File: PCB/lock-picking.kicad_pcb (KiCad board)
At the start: 2 copper layers, 25 x 24 mm, 22 parts, among them U1 HX PZ2.54-1X5P ZZ, U2 DRV8876PWPR, U3 MLX90393SLW-ABA-011-RE, U4 SMTSOM225BTR, U5 S2B-PH-K-S, U6 SMTSOM225BTR, U7 HX TYPE-C 16PIN, U8 AMS1117-5.0_C347223

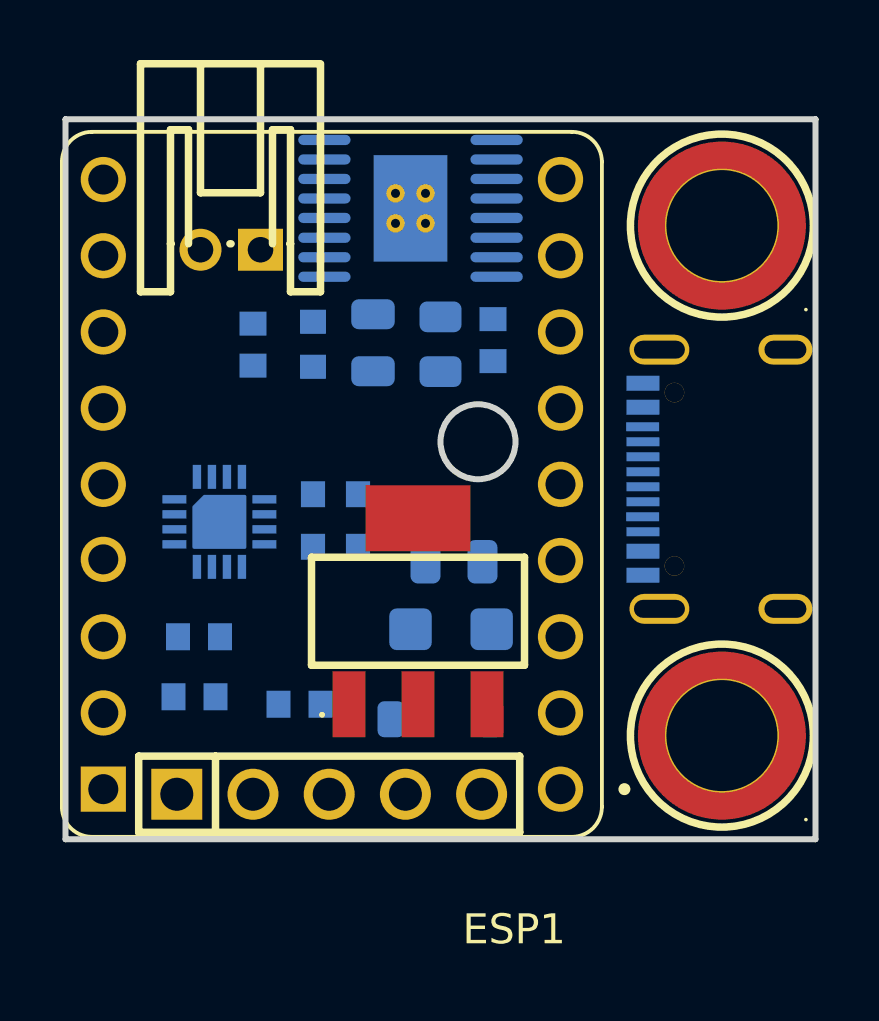
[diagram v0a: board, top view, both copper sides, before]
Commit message: PCB routing
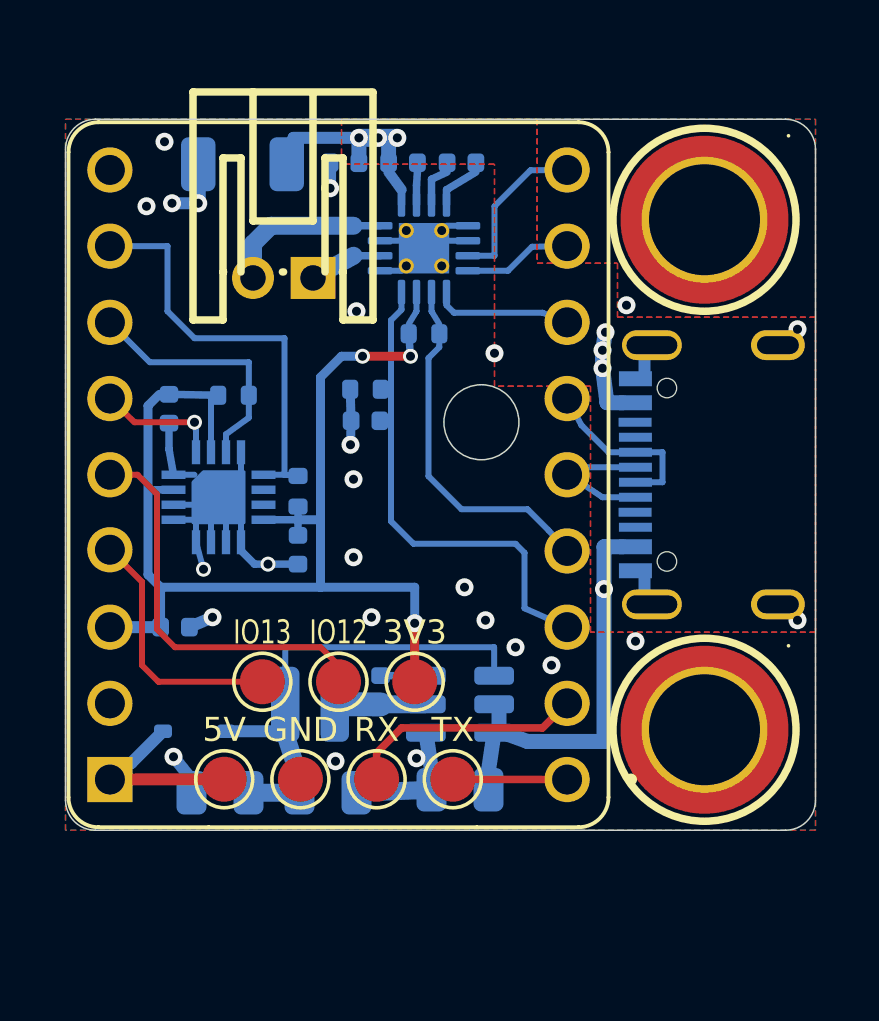
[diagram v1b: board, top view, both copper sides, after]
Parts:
- removed ESP1: ESP32-S3-SuperMini, footprints:ESP32-S3-SuperMini
- removed R5: 10, Resistor_SMD:R_0805_2012Metric
- removed U5: S2B-PH-K-S, EasyEDA:CONN-TH_S2B-PH-K-S-LF-SN
- removed U6: SMTSOM225BTR, EasyEDA:SMD_BD5.6-D3.6
- removed U7: HX TYPE-C 16PIN, EasyEDA:TYPE-C-SMD_HX-TYPE-C-16PIN
- removed U8: AMS1117-5.0_C347223, EasyEDA:SOT-223_L6.7-W3.5-P2.30-BR
- added C1: 10uF 25V, Capacitor_SMD:C_0805_2012Metric, B.Cu at (25.1, 34.4)
- added C10: 100nF 16V, Capacitor_SMD:C_0402_1005Metric, B.Cu at (19.8, 26.4)
- added C11: 10uF 6.3V, Capacitor_SMD:C_0402_1005Metric, B.Cu at (15.7, 28.9)
- added C12: 10nF 50V, Capacitor_SMD:C_0402_1005Metric, B.Cu at (22.0, 22.1)
- added H1: M2 SMD nut, Library:M2_SMD_nut_SMTSOM225_ring4.2, F.Cu at (33.3, 15.3)
- added H2: M2 SMD nut, Library:M2_SMD_nut_SMTSOM225_ring4.2, F.Cu at (33.3, 32.4)
- added J1: USB-C 16P (12V + I2C), Library:USB-C_HX-TYPE-C-16PIN_NPTH-pegs, B.Cu at (33.4, 23.9)
- added J2: Motor (JST-PH 2P), EasyEDA:CONN-TH_S2B-PH-K-S-LF-SN, F.Cu at (19.2, 17.3)
- added L1: 4.7uH, Inductor_SMD:L_Changjiang_FTC252012S, B.Cu at (20.1, 31.5)
- added R1: 1.5k 1%, Resistor_SMD:R_0402_1005Metric, B.Cu at (22.0, 21.0)
- added TP1: Pad, TestPoint:TestPoint_Pad_D1.5mm, F.Cu at (21.1, 30.8)
- added TP2: Pad, TestPoint:TestPoint_Pad_D1.5mm, F.Cu at (18.6, 30.8)
- added TP3: Pad, TestPoint:TestPoint_Pad_D1.5mm, F.Cu at (24.9, 34.0)
- added TP4: Pad, TestPoint:TestPoint_Pad_D1.5mm, F.Cu at (22.4, 34.0)
- added TP5: Pad, TestPoint:TestPoint_Pad_D1.5mm, F.Cu at (23.6, 30.8)
- added TP6: Pad, TestPoint:TestPoint_Pad_D1.5mm, F.Cu at (17.3, 34.0)
- added TP7: Pad, TestPoint:TestPoint_Pad_D1.5mm, F.Cu at (19.8, 34.0)
- C2, C9: value CC0603KRX7R9BB104 -> 100nF 16V; footprint EasyEDA:C0603 -> Capacitor_SMD:C_0402_1005Metric
- C3: value CL10B223KB8NNNC-22nF -> 47uF 6.3V; footprint EasyEDA:C0603 -> Capacitor_SMD:C_0805_2012Metric
- C4: value CC0603KRX7R9BB104 -> 47uF 6.3V; footprint EasyEDA:C0603 -> Capacitor_SMD:C_0805_2012Metric
- C5: value 10uF 25V -> 100nF 50V; footprint Capacitor_SMD:C_0805_2012Metric -> Capacitor_SMD:C_0402_1005Metric
- C6: value 10uF 16V tant -> 22uF 25V; footprint Capacitor_Tantalum_SMD:CP_EIA-3216-18_Kemet-A -> Capacitor_SMD:C_1206_3216Metric
- C7: value 10uF 25V -> 100nF 16V; footprint Capacitor_SMD:C_0805_2012Metric -> Capacitor_SMD:C_0402_1005Metric
- C8: value CC0603KRX7R9BB104 -> 22nF 50V; footprint EasyEDA:C0603 -> Capacitor_SMD:C_0402_1005Metric
- D1: value B5819W -> 1N5819WS; footprint Diode_SMD:D_SOD-123 -> Diode_SMD:D_SOD-323
- R2: value 0603WAF1501T5E -> 10k; footprint EasyEDA:R0603 -> Resistor_SMD:R_0402_1005Metric
- R3, R4: value 10k -> 2.2k; footprint EasyEDA:R0603 -> Resistor_SMD:R_0402_1005Metric
- U1: value HX PZ2.54-1X5P ZZ -> ESP32-S3-SuperMini; footprint EasyEDA:HDR-TH_5P-P2.54-V-M -> footprints:ESP32-S3-SuperMini
- U2: value DRV8876PWPR -> DRV8876RGTR; footprint EasyEDA:HTSSOP-16_L5.0-W4.4-P0.65-LS6.4-BL-EP -> Library:QFN-16-1EP_3x3mm_P0.5mm_EP1.68x1.68mm_ThermalVias0.3
- U4: value SMTSOM225BTR -> AP63205WU-7; footprint EasyEDA:SMD_BD5.6-D3.6 -> Package_TO_SOT_SMD:TSOT-23-6; moved to B.Cu
- moved C8 19.9 mm to (25.2, 13.4), turned to 0 degrees
- moved U4 18.2 mm to (25.1, 31.5), turned to 180 degrees
- moved C6 17.0 mm to (17.9, 13.5), turned to 180 degrees
- moved C3 16.1 mm to (20.8, 34.5), turned to 0 degrees
- moved C4 15.0 mm to (17.1, 34.5), turned to 180 degrees
- moved C7 13.4 mm to (23.2, 13.4)
- moved U1 10.7 mm to (21.1, 23.9), turned to 180 degrees
- moved D1 8.21 mm to (16.3, 32.4), turned to 0 degrees
- moved C9 7.67 mm to (15.4, 21.6), turned to -90 degrees
- moved R4 6.09 mm to (17.6, 21.2)
- moved C5 6.07 mm to (21.3, 13.4), turned to 180 degrees
- moved R2 3.72 mm to (23.9, 19.1), turned to 180 degrees
- moved C2 2.74 mm to (22.5, 31.0), turned to 90 degrees
- moved U2 1.40 mm to (23.9, 16.3)
- moved R3 1.25 mm to (19.8, 24.4), turned to -90 degrees
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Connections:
- C2 pad 1: 12v -> Net-(U4-SW)
- C2 pad 2: GND -> Net-(U4-BST)
- C3 pad 1: Net-(U2-CPL) -> +5V
- C3 pad 2: Net-(U2-CPH) -> GND
- C4 pad 1: Net-(U2-VCP) -> +5V
- C4 pad 2: 12v -> GND
- C5 pad 1: VIN_LDO -> +12V
- C6 pad 1: 5v -> +12V
- C7 pad 1: 12v -> /DRV_VCP
- C7 pad 2: GND -> +12V
- C8 pad 1: GND -> /DRV_CPH
- C8 pad 2: 3v3 -> /DRV_CPL
- C9 pad 1: GND -> +3V3
- C9 pad 2: 3v3 -> GND
- D1 pad 2: 5v -> +5V
- R2 pad 1: GND -> /DRV_nFAULT
- R2 pad 2: IPROPI -> +3V3
- R3 pad 1: 3v3 -> /MAG_SDA
- R3 pad 2: MAG_SDA -> +3V3
- R4 pad 1: 3v3 -> /MAG_SCL
- R4 pad 2: MAG_SCL -> +3V3
- U1 pad 1: VBUS -> /DRV_IPROPI
- U1 pad 2: GND -> /DRV_nFAULT
- U1 pad 3: GPIO9 -> /I2C_SDA
- U1 pad 4: GPIO8 -> /I2C_SCL
- U1 pad 5: GPIO7 -> /DRV_nSLEEP
- U2 pad 1: IN1 -> /DRV_nSLEEP
- U2 pad 10: Net-(U2-OUT2) -> /DRV_VCP
- U2 pad 11: 12v -> /DRV_CPH
- U2 pad 12: Net-(U2-VCP) -> /DRV_CPL
- U2 pad 13: Net-(U2-CPH) -> GND
- U2 pad 14: Net-(U2-CPL) -> GND
- U2 pad 15: GND -> /DRV_IN1_EN
- U2 pad 16: PMODE -> /DRV_IN2_PH
- U2 pad 2: IN2 -> /DRV_nFAULT
- U2 pad 3: nSLEEP -> +3V3
- U2 pad 4: nFAULT -> /DRV_IPROPI
- U2 pad 5: nSLEEP -> GND
- U2 pad 6: IPROPI -> /MOT_OUT1
- U2 pad 8: Net-(U2-OUT1) -> /MOT_OUT2
- U2 pad 9: GND -> +12V
- U3 pad 1: unconnected-(U3-INT-Pad1) -> /MAG_INT
- U3 pad 10: unconnected-(U3-N/C-Pad10) -> GND
- U3 pad 14: unconnected-(U3-N/C-Pad14) -> GND
- U3 pad 15: 3v3 -> +3V3
- U3 pad 16: unconnected-(U3-N/C-Pad16) -> GND
- U3 pad 17: unconnected-(U3-EP-Pad17) -> GND
- U3 pad 2: 3v3 -> +3V3
- U3 pad 3: MAG_SCL -> /MAG_SCL
- U3 pad 4: unconnected-(U3-N/C-Pad4) -> GND
- U3 pad 5: MAG_SDA -> /MAG_SDA
- U3 pad 8: 3v3 -> +3V3
- U3 pad 9: unconnected-(U3-N/C-Pad9) -> GND
- U4 pad 1: unconnected-(U4-Pad1)_1 -> +5V
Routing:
- net +3V3: track 0.00 -> 40.8 mm, vias 0 -> 3
- net GND: track 0.00 -> 26.1 mm, vias 0 -> 25
- net +12V: track 0.00 -> 22.9 mm, vias 0 -> 7
- net /DRV_IPROPI: track 0.00 -> 16.8 mm
- net /MAG_SDA: track 0.00 -> 14.1 mm
- net /EXP_IO12: track 0.00 -> 13.4 mm
- net +5V: track 0.00 -> 13.2 mm
- net /DRV_nFAULT: track 0.00 -> 11.7 mm
- net /MAG_SCL: track 0.00 -> 8.57 mm
- net /EXP_IO13: track 0.00 -> 8.53 mm
- net /EXP_RX: track 0.00 -> 7.91 mm
- net VBUS: track 0.00 -> 6.21 mm
- net /MOT_OUT2: track 0.00 -> 5.63 mm
- net /DRV_IN1_EN: track 0.00 -> 5.45 mm
- net /I2C_SCL: track 0.00 -> 4.78 mm
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- added copper zone on F.Cu, net +12V
- added copper zone on B.Cu, net GND
- added copper zone on F.Cu, net GND
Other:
- board size 25 x 24 mm -> 25 x 23.7 mm
- board text added: "3V3"
- board text added: "5V"
- board text added: "ESP socket keep out"
- board text added: "GND"
- board text added: "IO12"
- board text added: "IO13"
- board text added: "ROUTING NOTES rev 3b (2 layers, routed + poured, reviewed) Frame origin = board top-left (abs 12,12). Board 25.0 x 23.7, 1 mm corner radius. 1 BACK = every PCBA part + most signals. FRONT = GND pour, a 12 V copper area, short hops. 2 12 V: J1 top VBUS pad -> 3 vias -> front 12 V copper (gaps between ESP pins 6/5 and 5/4) -> inside the right header -> along the top edge -> 3 vias -> C5/C7/U2 VM. N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"
- board text added: "RX"
- board text added: "TX"
